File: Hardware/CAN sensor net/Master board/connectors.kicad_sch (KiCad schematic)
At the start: 18 parts, among them J1 Micro_SD_Card_Con, J2 USB_B_Micro, J3 Conn_02x05_SWD, J5 532610671, J6 532610671, J7 530470310, U2 USBLC6-2SC6

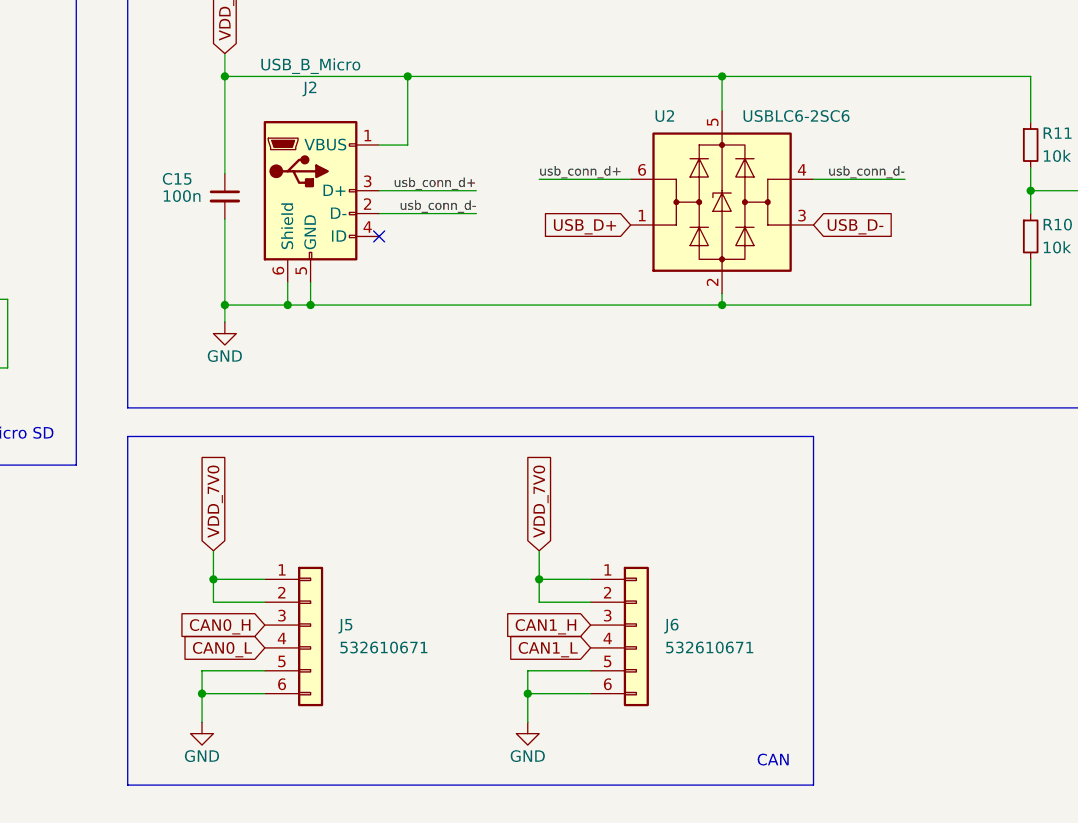
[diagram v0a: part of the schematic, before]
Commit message: Concept no trace
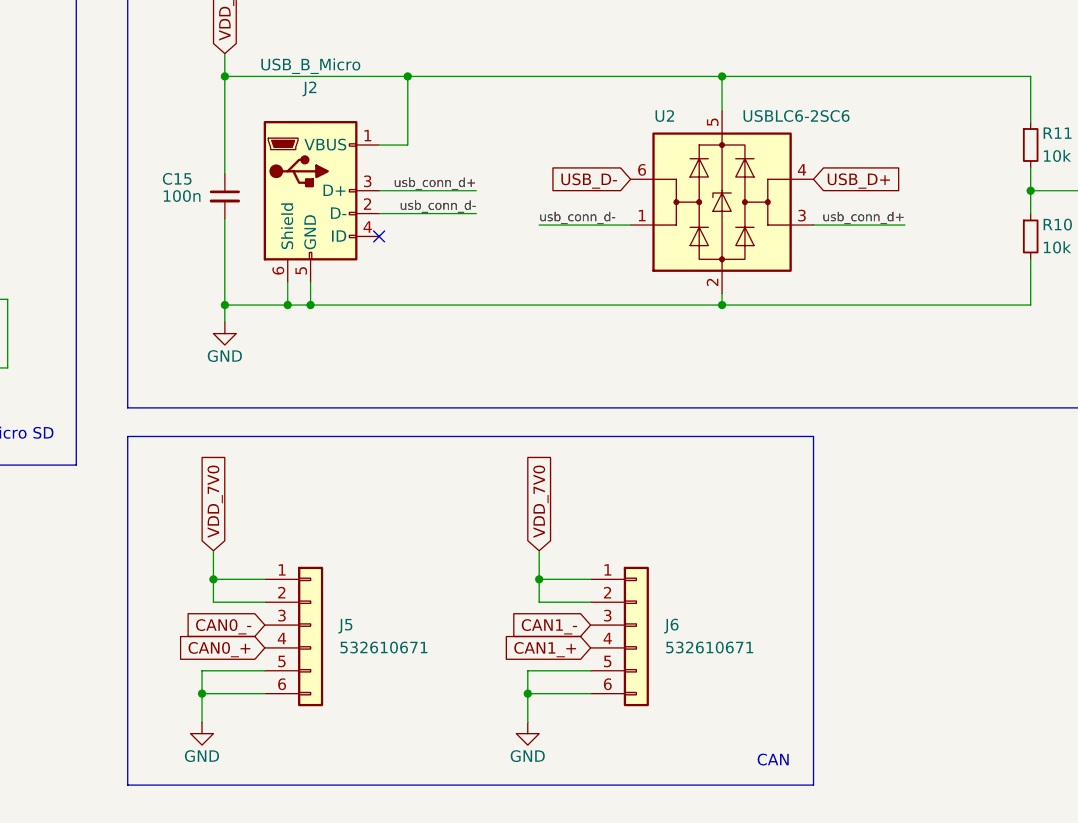
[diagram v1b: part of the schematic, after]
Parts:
- J7: footprint Connector_Molex:Molex_PicoBlade_53047-0310_1x03_P1.25mm_Vertical -> Connector_Molex:Molex_PicoBlade_53261-0371_1x03-1MP_P1.25mm_Horizontal
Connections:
- net USB_D+: now also U2.4 (I/O2); no longer U2.1 (I/O1)
- net USB_D-: now also U2.6 (I/O1); no longer U2.3 (I/O2)
- net usb_conn_d+: now also U2.3 (I/O2); no longer U2.6 (I/O1)
- net usb_conn_d-: now also U2.1 (I/O1); no longer U2.4 (I/O2)
- net CAN0_H renamed CAN0_-
- net CAN0_L renamed CAN0_+
- net CAN1_H renamed CAN1_-
- net CAN1_L renamed CAN1_+
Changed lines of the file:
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@@
-	(wire
-		(pts
-			(xy 207.645 50.8) (xy 197.485 50.8)
-		)
-		(stroke
-			(width 0)
-			(type default)
-		)
-	)
 	(wire
 		(pts
@@
 	(wire
 		(pts
+			(xy 238.125 55.88) (xy 227.965 55.88)
+		)
+		(stroke
+			(width 0)
+			(type default)
+		)
+	)
+	(wire
+		(pts
 			(xy 76.835 39.37) (xy 76.835 41.275)
 		)
@@
 	(wire
 		(pts
-			(xy 238.125 50.8) (xy 227.965 50.8)
-		)
-		(stroke
-			(width 0)
-			(type default)
-		)
-	)
-	(wire
-		(pts
 			(xy 53.975 33.02) (xy 53.975 34.29)
 		)
@@
 		(pts
 			(xy 34.29 43.815) (xy 69.215 43.815)
+		)
+		(stroke
+			(width 0)
+			(type default)
+		)
+	)
+	(wire
+		(pts
+			(xy 197.485 55.88) (xy 207.645 55.88)
 		)
 		(stroke
@@
 	)
 	(label "usb_conn_d+"
-		(at 197.485 50.8 0)
+		(at 238.125 55.88 180)
 		(fields_autoplaced yes)
 		(effects
@@
 				(size 1 1)
 			)
+			(justify right bottom)
+		)
+	)
+	(label "usb_conn_d-"
+		(at 197.485 55.88 0)
+		(fields_autoplaced yes)
+		(effects
+			(font
+				(size 1 1)
+			)
 			(justify left bottom)
-		)
-	)
-	(label "usb_conn_d-"
-		(at 238.125 50.8 180)
-		(fields_autoplaced yes)
-		(effects
-			(font
-				(size 1 1)
-			)
-			(justify right bottom)
 		)
 	)
@@
 		)
 	)
-	(global_label "CAN0_L"
+	(global_label "CAN0_-"
 		(shape input)
-		(at 167.005 102.87 180)
+		(at 167.005 100.33 180)
 		(fields_autoplaced yes)
 		(effects
@@
 		)
 		(property "Intersheetrefs" "${INTERSHEET_REFS}"
-			(at 157.1255 102.87 0)
+			(at 156.5812 100.33 0)
 			(effects
 				(font
@@
 		)
 	)
+	(global_label "CAN1_+"
+		(shape input)
+		(at 203.2 102.87 180)
+		(fields_autoplaced yes)
+		(effects
+			(font
+				(size 1.27 1.27)
+			)
+			(justify right)
+		)
+		(property "Intersheetrefs" "${INTERSHEET_REFS}"
+			(at 192.7762 102.87 0)
+			(effects
+				(font
+					(size 1.27 1.27)
+				)
+				(justify right)
+				(hide yes)
+			)
+		)
+	)
 	(global_label "VDD_3V3"
 		(shape input)
@@
 	(global_label "USB_D+"
 		(shape input)
-		(at 207.645 55.88 180)
+		(at 227.965 50.8 0)
 		(fields_autoplaced yes)
 		(effects
@@
 				(size 1.27 1.27)
 			)
-			(justify right)
+			(justify left)
 		)
 		(property "Intersheetrefs" "${INTERSHEET_REFS}"
-			(at 197.0398 55.88 0)
-			(effects
-				(font
-					(size 1.27 1.27)
-				)
-				(justify right)
+			(at 238.5702 50.8 0)
+			(effects
+				(font
+					(size 1.27 1.27)
+				)
+				(justify left)
 				(hide yes)
 			)
@@
 		)
 	)
-	(global_label "CAN1_L"
-		(shape input)
-		(at 203.2 102.87 180)
-		(fields_autoplaced yes)
-		(effects
-			(font
-				(size 1.27 1.27)
-			)
-			(justify right)
-		)
-		(property "Intersheetrefs" "${INTERSHEET_REFS}"
-			(at 193.3205 102.87 0)
-			(effects
-				(font
-					(size 1.27 1.27)
-				)
-				(justify right)
-				(hide yes)
-			)
-		)
-	)
-	(global_label "USB_D-"
-		(shape input)
-		(at 227.965 55.88 0)
-		(fields_autoplaced yes)
-		(effects
-			(font
-				(size 1.27 1.27)
-			)
-			(justify left)
-		)
-		(property "Intersheetrefs" "${INTERSHEET_REFS}"
-			(at 238.5702 55.88 0)
-			(effects
-				(font
-					(size 1.27 1.27)
-				)
-				(justify left)
-				(hide yes)
-			)
-		)
-	)
-	(global_label "CAN1_H"
+	(global_label "CAN1_-"
 		(shape input)
 		(at 203.2 100.33 180)
@@
 		)
 		(property "Intersheetrefs" "${INTERSHEET_REFS}"
-			(at 193.0181 100.33 0)
+			(at 192.7762 100.33 0)
 			(effects
 				(font
@@
 		)
 	)
-	(global_label "CAN0_H"
+	(global_label "USB_D-"
 		(shape input)
-		(at 167.005 100.33 180)
+		(at 207.645 50.8 180)
 		(fields_autoplaced yes)
 		(effects
@@
 		)
 		(property "Intersheetrefs" "${INTERSHEET_REFS}"
-			(at 156.8231 100.33 0)
+			(at 197.0398 50.8 0)
+			(effects
+				(font
+					(size 1.27 1.27)
+				)
+				(justify right)
+				(hide yes)
+			)
+		)
+	)
+	(global_label "CAN0_+"
+		(shape input)
+		(at 167.005 102.87 180)
+		(fields_autoplaced yes)
+		(effects
+			(font
+				(size 1.27 1.27)
+			)
+			(justify right)
+		)
+		(property "Intersheetrefs" "${INTERSHEET_REFS}"
+			(at 156.5812 102.87 0)
 			(effects
 				(font
@@
 			)
 		)
-		(property "Footprint" "Connector_Molex:Molex_PicoBlade_53047-0310_1x03_P1.25mm_Vertical"
+		(property "Footprint" "Connector_Molex:Molex_PicoBlade_53261-0371_1x03-1MP_P1.25mm_Horizontal"
 			(at 169.545 132.08 0)
 			(effects

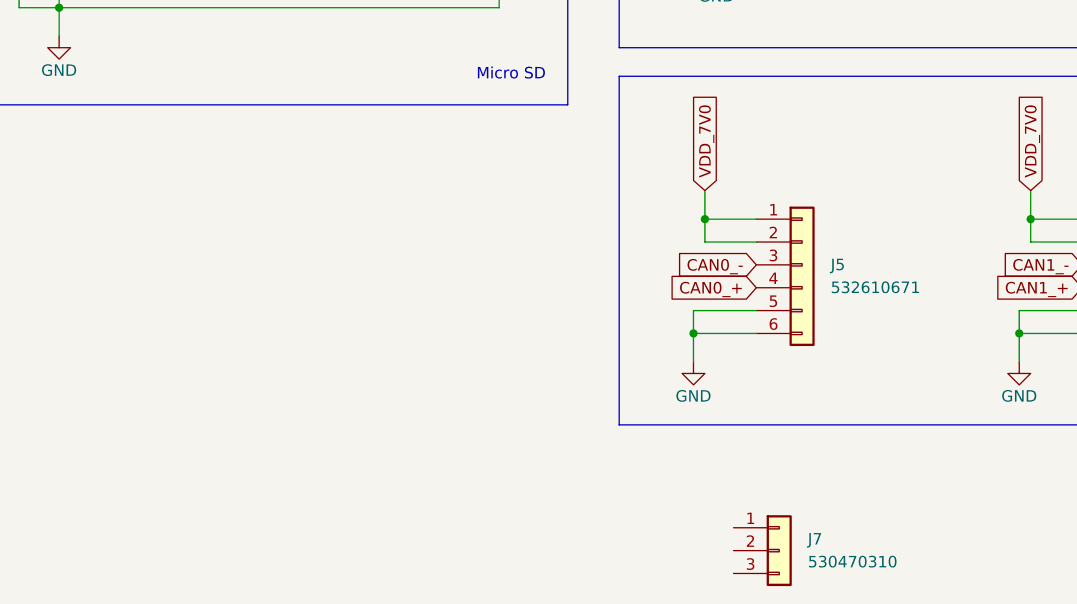
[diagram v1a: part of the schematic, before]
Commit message: added band pass filter to piezo board
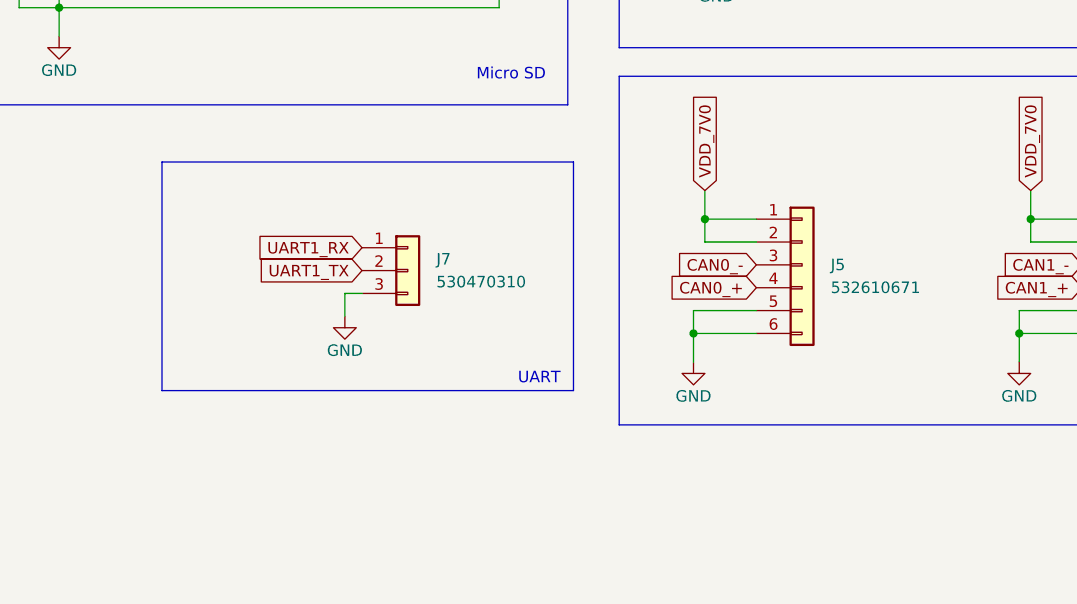
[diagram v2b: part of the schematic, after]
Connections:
- net GND: now also J7.3 (Pin_3)
- net UART1_RX: now reaches J7.1 (Pin_1)
- net UART1_TX: now reaches J7.2 (Pin_2)
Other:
- note added: "UART"
- moved on the sheet: J7
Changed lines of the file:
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@@
 	(wire
 		(pts
+			(xy 121.285 103.505) (xy 121.285 106.045)
+		)
+		(stroke
+			(width 0)
+			(type default)
+		)
+	)
+	(wire
+		(pts
 			(xy 76.835 39.37) (xy 76.835 41.275)
 		)
@@
 		)
 	)
+	(polyline
+		(pts
+			(xy 100.965 88.9) (xy 146.685 88.9)
+		)
+		(stroke
+			(width 0)
+			(type default)
+		)
+	)
 	(wire
 		(pts
@@
 		)
 	)
+	(polyline
+		(pts
+			(xy 100.965 114.3) (xy 146.685 114.3)
+		)
+		(stroke
+			(width 0)
+			(type default)
+		)
+	)
 	(wire
 		(pts
@@
 	(wire
 		(pts
+			(xy 123.19 103.505) (xy 121.285 103.505)
+		)
+		(stroke
+			(width 0)
+			(type default)
+		)
+	)
+	(wire
+		(pts
 			(xy 196.215 111.125) (xy 196.215 107.95)
 		)
@@
 		)
 	)
+	(polyline
+		(pts
+			(xy 146.685 88.9) (xy 146.685 114.3)
+		)
+		(stroke
+			(width 0)
+			(type default)
+		)
+	)
 	(wire
 		(pts
@@
 		)
 	)
+	(polyline
+		(pts
+			(xy 100.965 114.3) (xy 100.965 88.9)
+		)
+		(stroke
+			(width 0)
+			(type default)
+		)
+	)
 	(wire
 		(pts
@@
 		)
 	)
+	(text "UART"
+		(exclude_from_sim no)
+		(at 142.875 113.03 0)
+		(effects
+			(font
+				(size 1.27 1.27)
+			)
+		)
+	)
 	(text "SWD (Debug)"
 		(exclude_from_sim no)
@@
 		)
 	)
+	(global_label "UART1_TX"
+		(shape input)
+		(at 123.19 100.965 180)
+		(fields_autoplaced yes)
+		(effects
+			(font
+				(size 1.27 1.27)
+			)
+			(justify right)
+		)
+		(property "Intersheetrefs" "${INTERSHEET_REFS}"
+			(at 111.1939 100.965 0)
+			(effects
+				(font
+					(size 1.27 1.27)
+				)
+				(justify right)
+				(hide yes)
+			)
+		)
+	)
 	(global_label "DEBUG_SWDIO"
 		(shape input)
@@
 		)
 	)
+	(global_label "UART1_RX"
+		(shape input)
+		(at 123.19 98.425 180)
+		(fields_autoplaced yes)
+		(effects
+			(font
+				(size 1.27 1.27)
+			)
+			(justify right)
+		)
+		(property "Intersheetrefs" "${INTERSHEET_REFS}"
+			(at 110.8915 98.425 0)
+			(effects
+				(font
+					(size 1.27 1.27)
+				)
+				(justify right)
+				(hide yes)
+			)
+		)
+	)
 	(global_label "VDD_3V3"
 		(shape input)
@@
 	)
 	(symbol
+		(lib_name "GND_1")
+		(lib_id "power:GND")
+		(at 121.285 106.045 0)
+		(unit 1)
+		(exclude_from_sim no)
+		(in_bom yes)
+		(on_board yes)
+		(dnp no)
+		(property "Reference" "#PWR09"
+			(at 121.285 112.395 0)
+			(effects
+				(font
+					(size 1.27 1.27)
+				)
+				(hide yes)
+			)
+		)
+		(property "Value" "GND"
+			(at 121.285 109.855 0)
+			(effects
+				(font
+					(size 1.27 1.27)
+				)
+			)
+		)
+		(property "Footprint" ""
+			(at 121.285 106.045 0)
+			(effects
+				(font
+					(size 1.27 1.27)
+				)
+				(hide yes)
+			)
+		)
+		(property "Datasheet" ""
+			(at 121.285 106.045 0)
+			(effects
+				(font
+					(size 1.27 1.27)
+				)
+				(hide yes)
+			)
+		)
+		(property "Description" "Power symbol creates a global label with name \"GND\" , ground"
+			(at 121.285 106.045 0)
+			(effects
+				(font
+					(size 1.27 1.27)
+				)
+				(hide yes)
+			)
+		)
+		(pin "1"
+		)
+		(instances
+			(project "Master board"
+				(path "/11ca9491-ebda-4c18-be98-3e552caaabb4/b817a2d8-bdd2-4de0-9d33-c531bafe0dc5"
+					(reference "#PWR09")
+					(unit 1)
+				)
+			)
+		)
+	)
+	(symbol
 		(lib_id "power:GND")
 		(at 196.215 111.125 0)
@@
 	(symbol
 		(lib_id "Connector_Generic:Conn_01x03")
-		(at 169.545 132.08 0)
+		(at 128.27 100.965 0)
 		(unit 1)
 		(exclude_from_sim no)
@@
 		(fields_autoplaced yes)
 		(property "Reference" "J7"
-			(at 172.72 130.8099 0)
+			(at 131.445 99.6949 0)
 			(effects
 				(font
@@
 		)
 		(property "Value" "530470310"
-			(at 172.72 133.3499 0)
+			(at 131.445 102.2349 0)
 			(effects
 				(font
@@
 		)
 		(property "Footprint" "Connector_Molex:Molex_PicoBlade_53261-0371_1x03-1MP_P1.25mm_Horizontal"
-			(at 169.545 132.08 0)
+			(at 128.27 100.965 0)
 			(effects
 				(font
@@
 		)
 		(property "Datasheet" "~"
-			(at 169.545 132.08 0)
+			(at 128.27 100.965 0)
 			(effects
 				(font
@@
 		)
 		(property "Description" "Generic connector, single row, 01x03, script generated (kicad-library-utils/schlib/autogen/connector/)"
-			(at 169.545 132.08 0)
+			(at 128.27 100.965 0)
 			(effects
 				(font

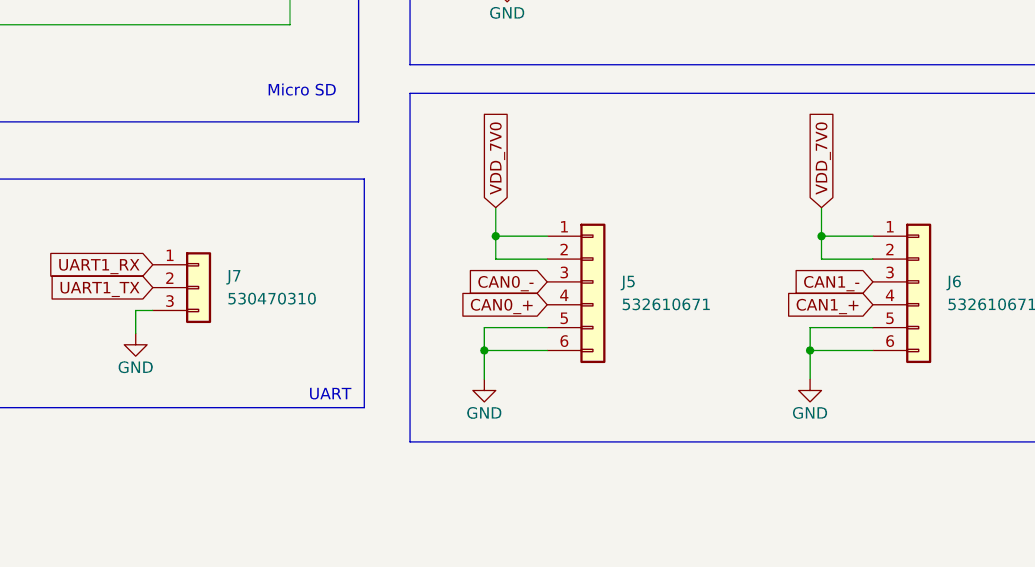
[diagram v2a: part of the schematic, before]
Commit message: Pre-production
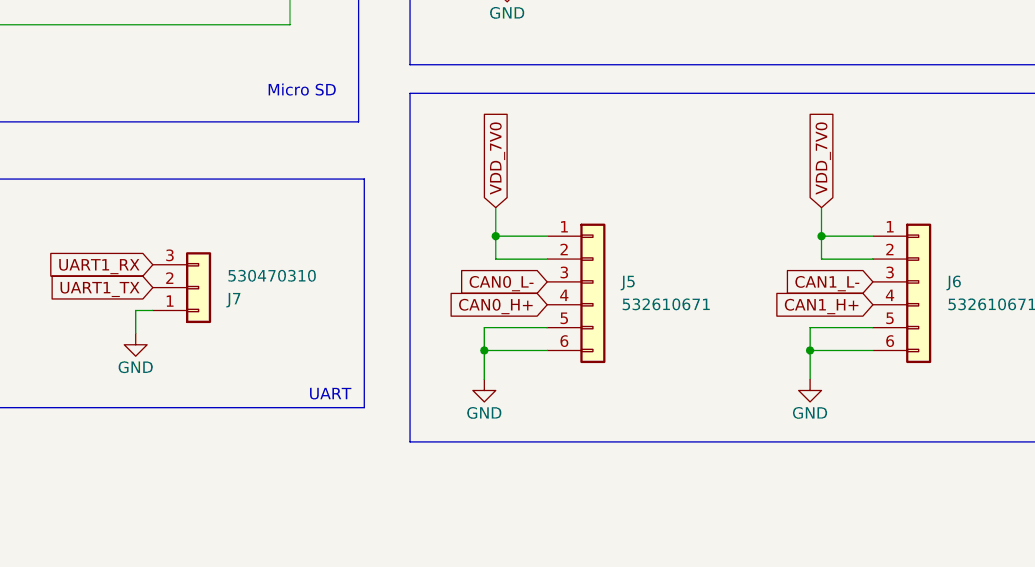
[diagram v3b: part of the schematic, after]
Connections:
- net GND: now also J7.1 (Pin_1); no longer J7.3 (Pin_3)
- net UART1_RX: now also J7.3 (Pin_3); no longer J7.1 (Pin_1)
- net CAN0_+ renamed CAN0_H+
- net CAN0_- renamed CAN0_L-
- net CAN1_+ renamed CAN1_H+
- net CAN1_- renamed CAN1_L-
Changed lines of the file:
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@@
 		)
 	)
-	(global_label "CAN0_-"
+	(global_label "CAN0_L-"
 		(shape input)
 		(at 167.005 100.33 180)
@@
 		)
 		(property "Intersheetrefs" "${INTERSHEET_REFS}"
-			(at 156.5812 100.33 0)
+			(at 155.5531 100.33 0)
 			(effects
 				(font
@@
 		)
 	)
-	(global_label "CAN1_+"
+	(global_label "CAN1_H+"
 		(shape input)
 		(at 203.2 102.87 180)
@@
 		)
 		(property "Intersheetrefs" "${INTERSHEET_REFS}"
-			(at 192.7762 102.87 0)
+			(at 191.4457 102.87 0)
 			(effects
 				(font
@@
 		)
 	)
-	(global_label "CAN1_-"
+	(global_label "CAN1_L-"
 		(shape input)
 		(at 203.2 100.33 180)
@@
 		)
 		(property "Intersheetrefs" "${INTERSHEET_REFS}"
-			(at 192.7762 100.33 0)
+			(at 191.7481 100.33 0)
 			(effects
 				(font
@@
 		)
 	)
-	(global_label "CAN0_+"
+	(global_label "CAN0_H+"
 		(shape input)
 		(at 167.005 102.87 180)
@@
 		)
 		(property "Intersheetrefs" "${INTERSHEET_REFS}"
-			(at 156.5812 102.87 0)
+			(at 155.2507 102.87 0)
 			(effects
 				(font
@@
 		(lib_id "Connector_Generic:Conn_01x03")
 		(at 128.27 100.965 0)
-		(unit 1)
-		(exclude_from_sim no)
-		(in_bom yes)
-		(on_board yes)
-		(dnp no)
-		(fields_autoplaced yes)
+		(mirror x)
+		(unit 1)
+		(exclude_from_sim no)
+		(in_bom yes)
+		(on_board yes)
+		(dnp no)
 		(property "Reference" "J7"
-			(at 131.445 99.6949 0)
+			(at 131.445 102.2351 0)
 			(effects
 				(font
@@
 		)
 		(property "Value" "530470310"
-			(at 131.445 102.2349 0)
-			(effects
-				(font
+			(at 131.445 99.6951 0)
+			(effects
+				(font
